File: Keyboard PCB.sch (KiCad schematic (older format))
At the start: 150 parts, among them J1 Connector_Generic_Conn_01x04, SW1 SW_Push, U1 ATmega32U4-AU, Y1 16MHz

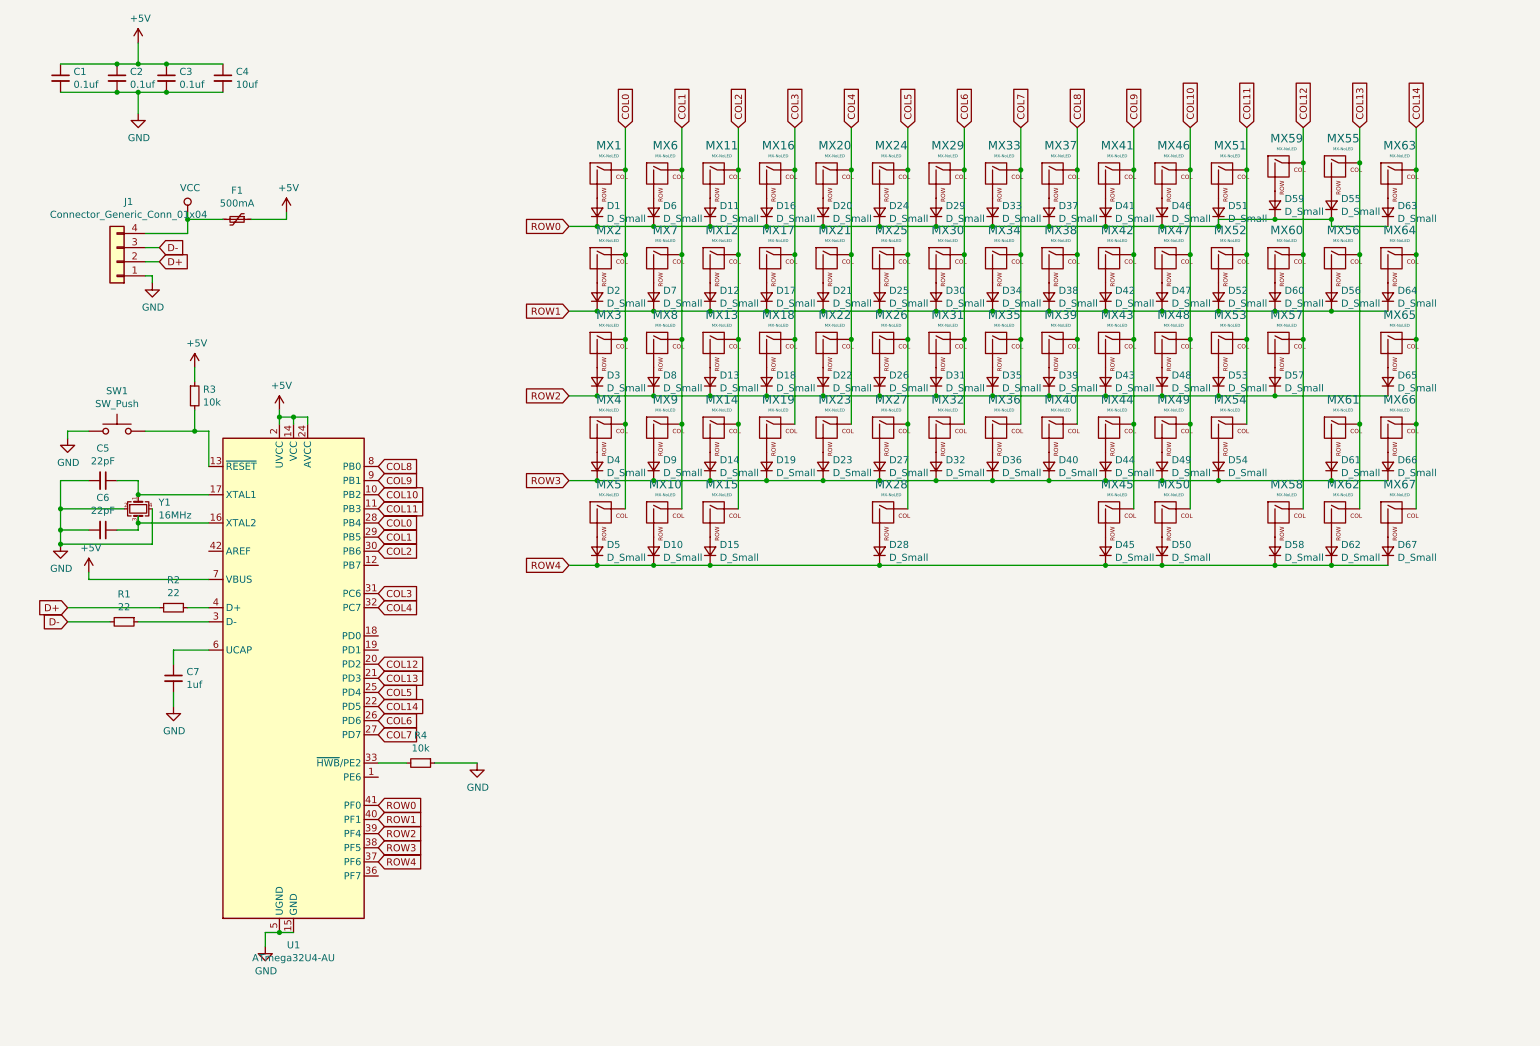
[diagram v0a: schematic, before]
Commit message: Final keyboard file extraction
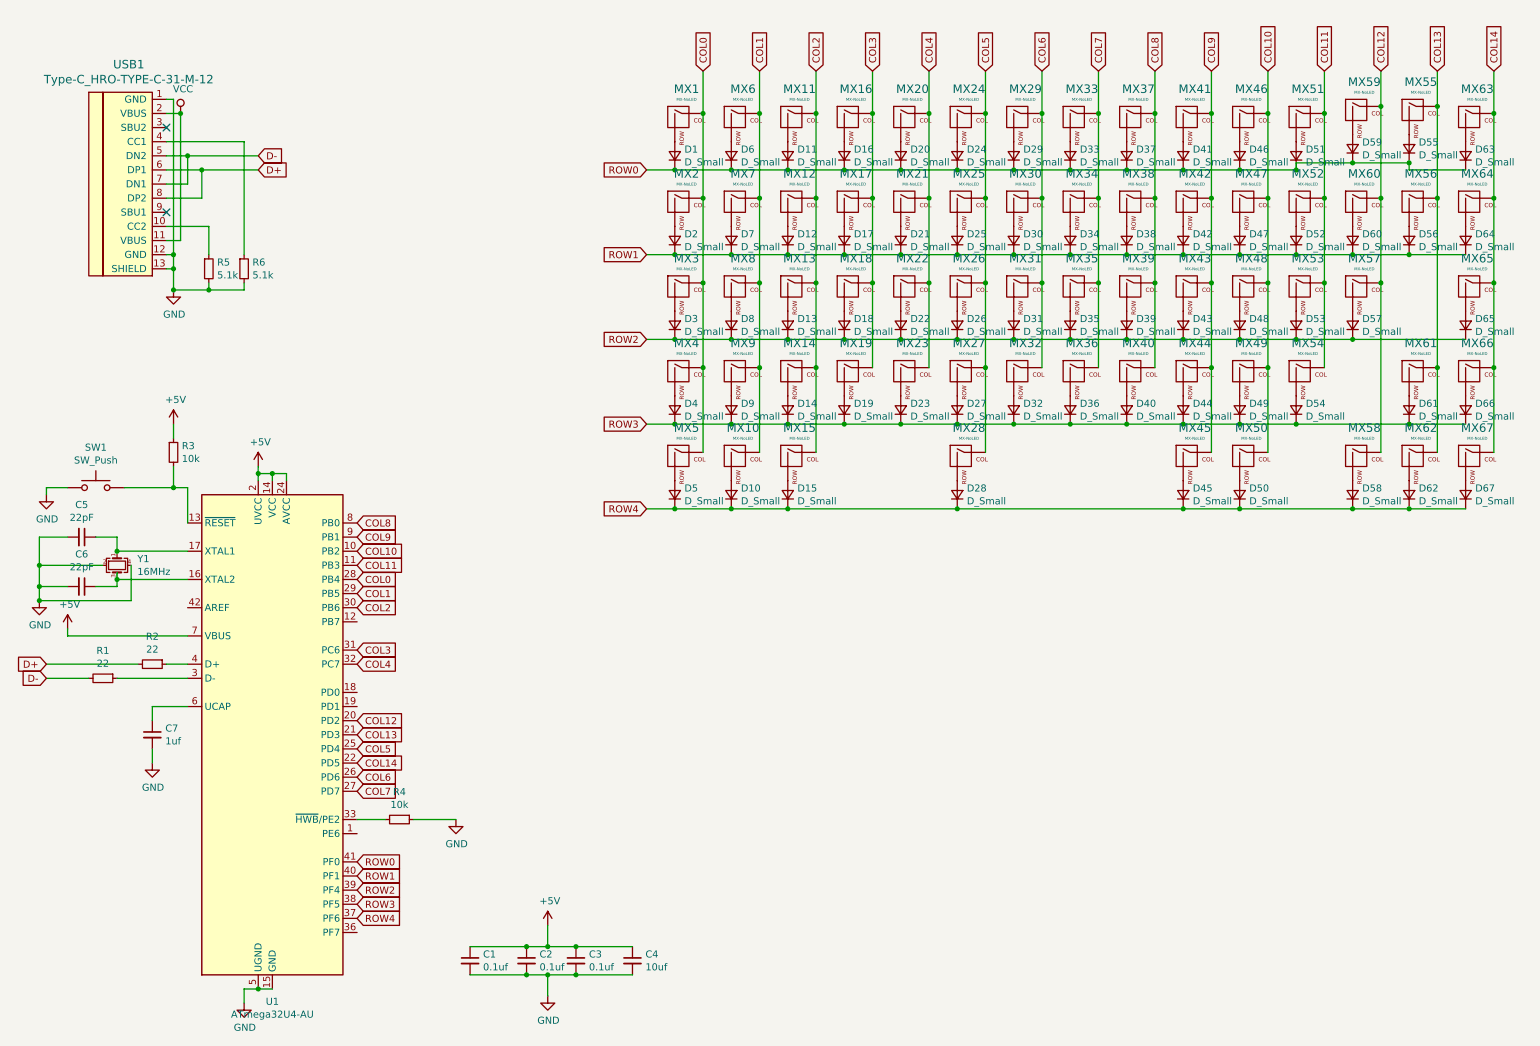
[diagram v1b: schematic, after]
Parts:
- removed F1: 500mA, Fuse:Fuse_1206_3216Metric_Pad1.42x1.75mm_HandSolder, symbol Device:Polyfuse_Small
- removed J1: Connector_Generic_Conn_01x04, Connector_JST:JST_ZE_SM04B-ZESS-TB_1x04-1MP_P1.50mm_Horizontal, symbol Unified-Daughterboard-cache:Connector_Generic_Conn_01x04
- added R5, R6: 5.1k, Resistor_SMD:R_0805_2012Metric_Pad1.15x1.40mm_HandSolder, symbol Device:R_Small
- added USB1: Type-C_HRO-TYPE-C-31-M-12, Type-C:HRO-TYPE-C-31-M-12-HandSoldering, symbol Unified-Daughterboard-cache:Type-C_HRO-TYPE-C-31-M-12
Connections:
- net D+: now also USB1.6 (DP1), USB1.8 (DP2)
- net D-: now also USB1.5 (DN2), USB1.7 (DN1)
- net GND: now also R5.2, R6.2, USB1.1 (GND), USB1.12 (GND), USB1.13 (SHIELD)
- net VCC: now also USB1.11 (VBUS), USB1.2 (VBUS)
- new net: R5.1, USB1.10 (CC2)
- new net: R6.1, USB1.4 (CC1)
- no-connect marks 0 -> 2
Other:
- moved on the sheet: C1, C2, C3, C4, C5, C6, C7, D1, D10, D11, D12, D13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
